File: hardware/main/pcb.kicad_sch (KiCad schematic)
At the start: 11 parts, among them J3 Conn_01x03_Socket

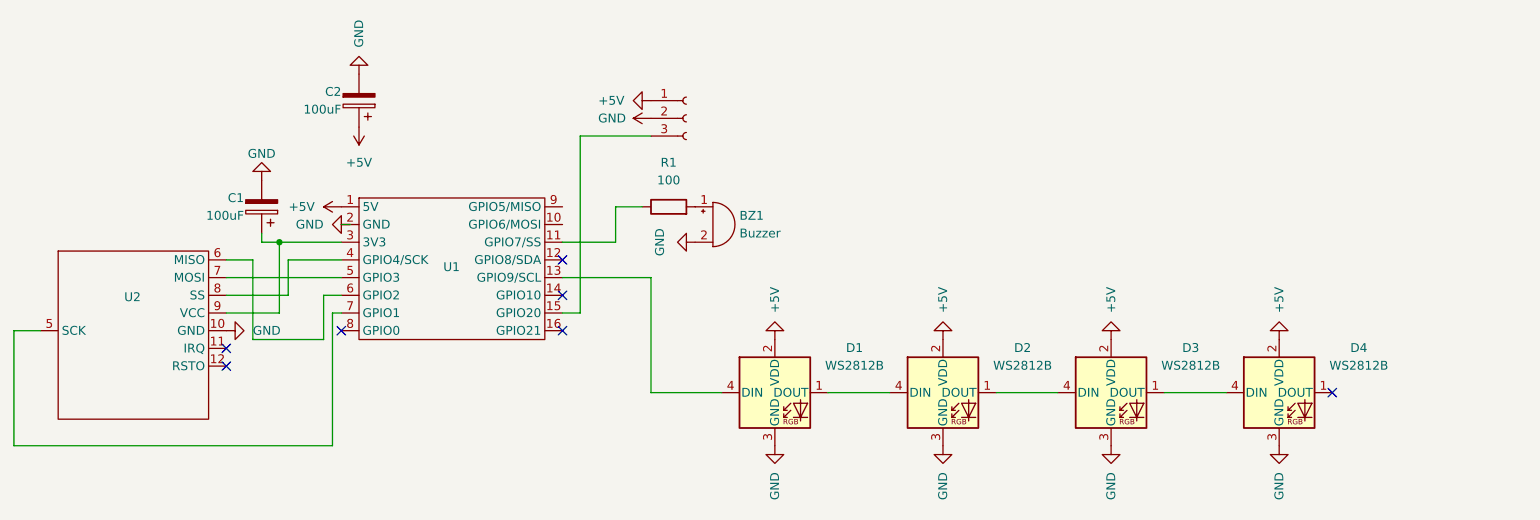
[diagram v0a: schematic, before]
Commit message: add capasitors to led
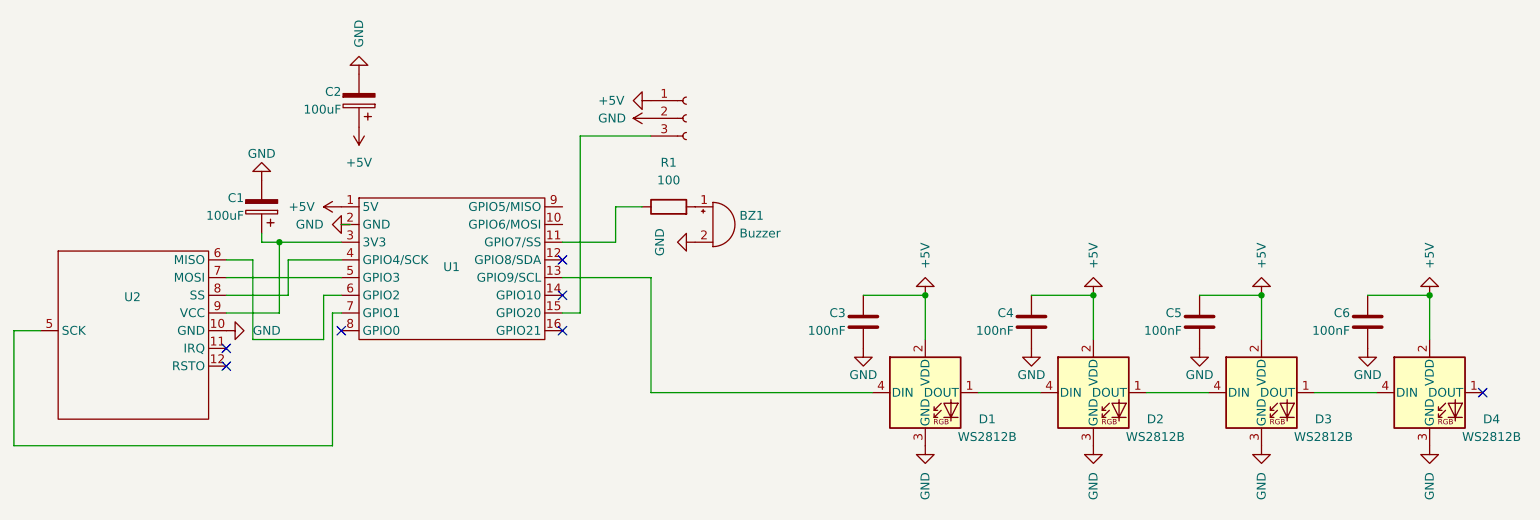
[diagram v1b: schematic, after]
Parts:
- added C3, C4, C5, C6: 100nF, prismo:C_Disc_D3.0mm_W1.6mm_P2.50mm, symbol prismo:C
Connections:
- net +5V: now also C3.1, C4.1, C5.1, C6.1
- net GND: now also C3.2, C4.2, C5.2, C6.2
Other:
- moved on the sheet: D1, D2, D3, D4
